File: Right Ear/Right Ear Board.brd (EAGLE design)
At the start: 157.5 x 20.3 mm, 6 parts, among them J1 502585-0470

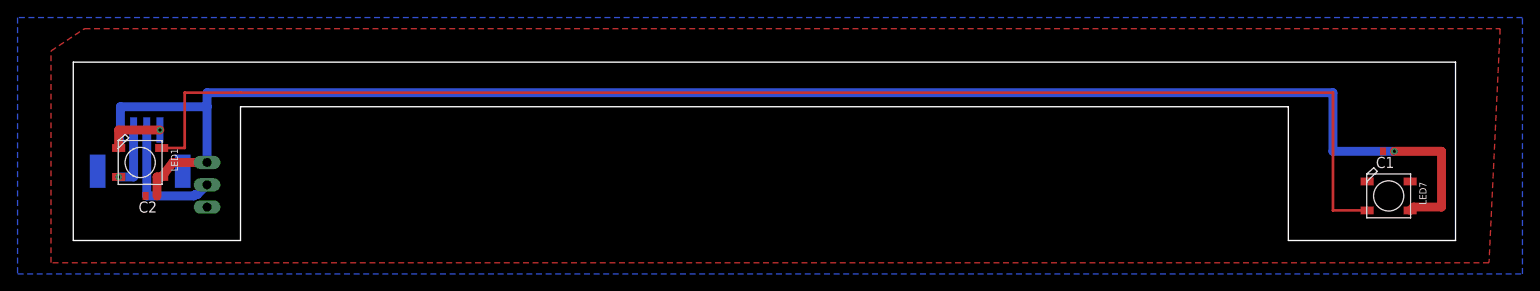
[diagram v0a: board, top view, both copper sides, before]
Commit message: Update right ear boards
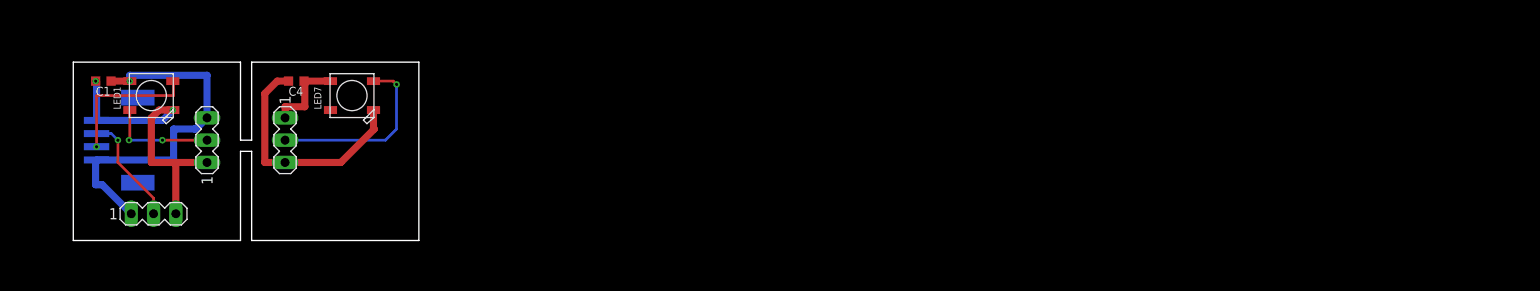
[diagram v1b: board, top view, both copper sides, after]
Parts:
- removed C2: (no value), rcl:C0402
- added C4: 10uF, rcl:C0603K
- added SV2, SV3: (no value), con-lstb:MA03-1
- C1: value (none) -> 10uF; device rcl:C0402 -> rcl:C0603K
- moved C1 146.6 mm to (3.43, 18.2)
- moved LED7 118.7 mm to (31.8, 16.5), turned to 180 degrees
- moved LED1 7.73 mm to (8.89, 16.5), turned to 180 degrees
- moved SV1 6.93 mm to (9.14, 3.05), flipped to the top, turned to 0 degrees
- moved J1 2.84 mm to (6.35, 11.4), turned to 270 degrees
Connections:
- removed net N$1: LED1.2-DOUT, LED7.4-DIN
- new net DATA: LED1.2-DOUT, LED7.4-DIN, SV2.2, SV3.2
- net +5V: now also C4.1, SV2.1, SV3.3; no longer C2.1
- net GND: now also C4.2, SV2.3, SV3.1; no longer C2.2
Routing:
- net N$1: track 157.1 -> 0.00 mm
- net +5V: track 186.5 -> 50.9 mm
- net GND: track 6.75 -> 61.3 mm, vias 1 -> 2
- net DATA: track 0.00 -> 33.5 mm, vias 0 -> 3
- net DI: track 7.05 -> 16.3 mm
- net SERVO_PWM: track 14.9 -> 12.8 mm, vias 0 -> 1
- removed copper zone on layer 1, net GND
- removed copper zone on layer 16, net GND
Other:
- board size 157.5 x 20.3 mm -> 39.4 x 20.3 mm
